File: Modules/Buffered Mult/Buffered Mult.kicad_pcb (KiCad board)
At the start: 2 copper layers, 50 x 200 mm, 20 parts

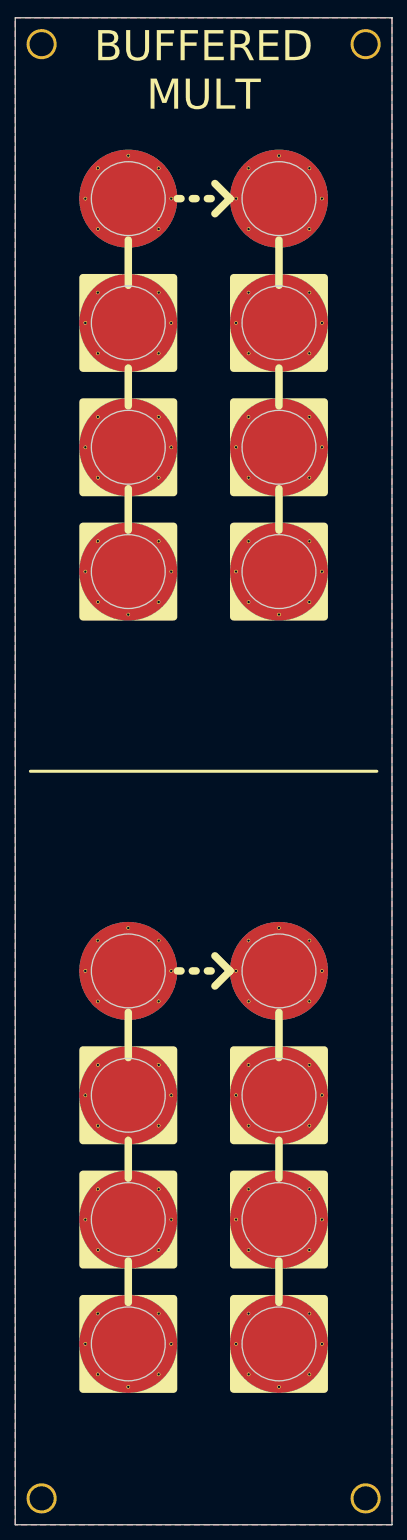
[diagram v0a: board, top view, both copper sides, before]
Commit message: Testing out gerber generation
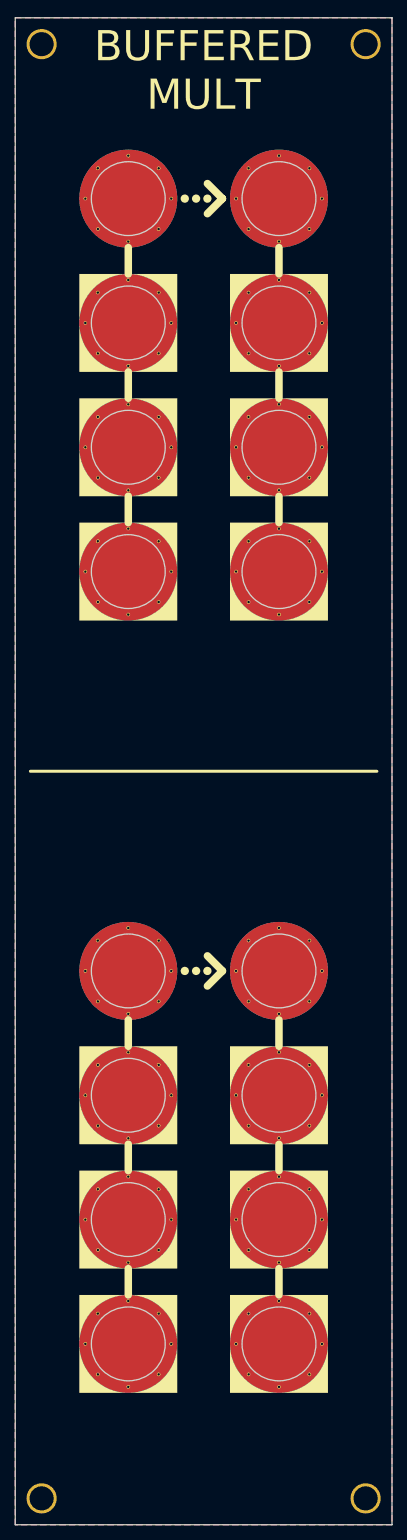
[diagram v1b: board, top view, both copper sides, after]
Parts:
- H10, H11, H12, H15, H16, H17, H18, H19, H20, H7, H8, H9: footprint SynthStuff:Jack_6.35mm_Cutout_Output_v2 -> SynthStuff:Jack_6.35mm_Cutout_Output_v4
